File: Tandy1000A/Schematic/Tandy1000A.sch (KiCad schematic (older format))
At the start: 19 parts, among them J5 Floppy, U12 74LS138, U17 8259A, U25 VC2587/8079011 Custom, U26 74LS244, U28 8088, U31 74LS04, U41 74LS244, U51 BIOS ROM, U58 7417, U9 TACO111/3A-2125-BB/8079012 Cu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

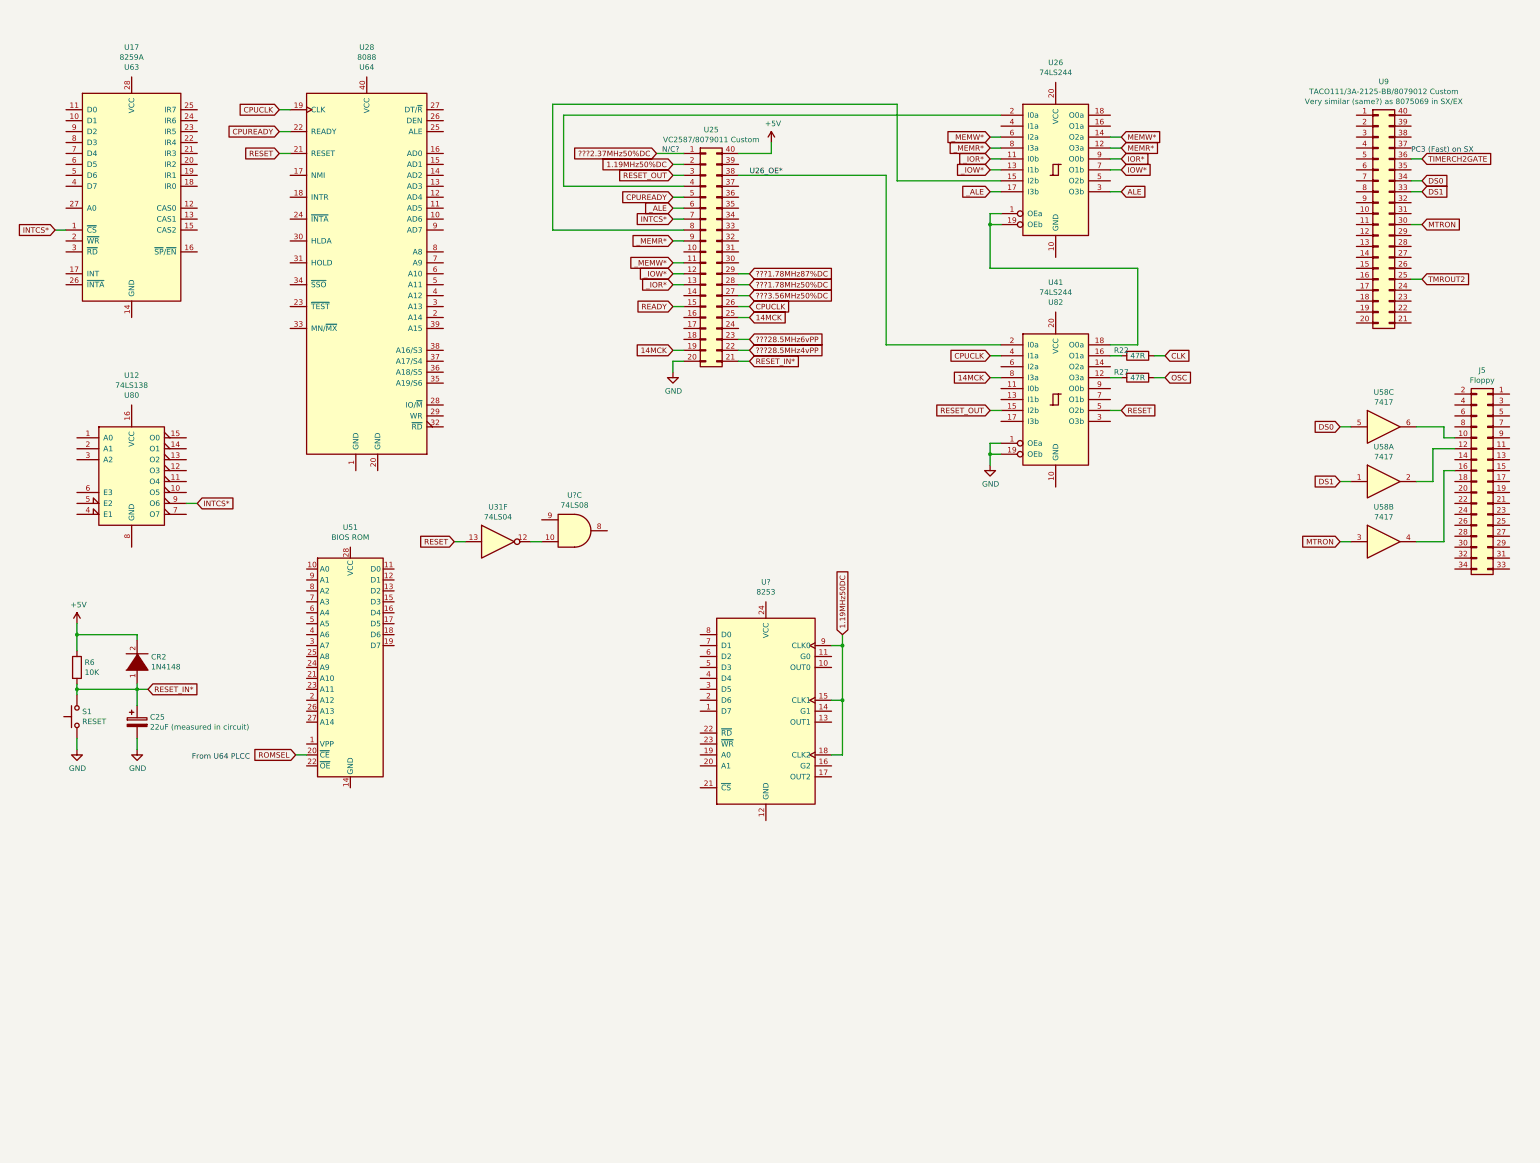
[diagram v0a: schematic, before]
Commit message: Readme and schematic updates.
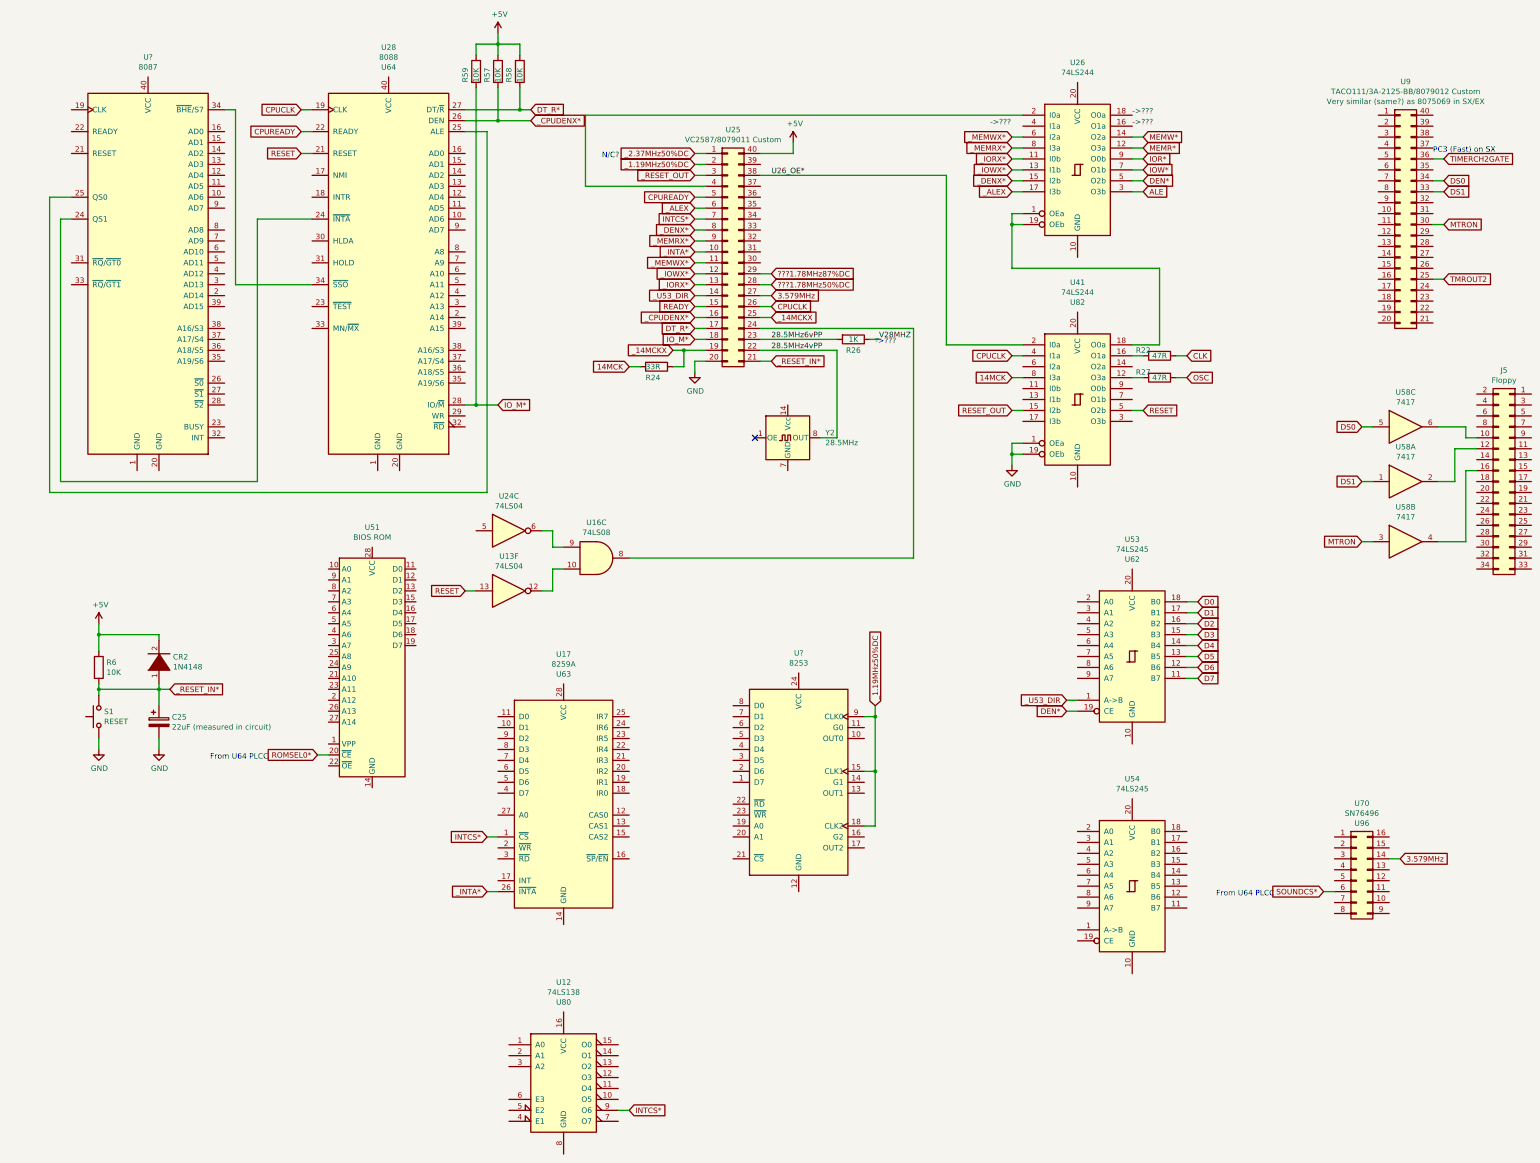
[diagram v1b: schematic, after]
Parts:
- added R24: 33R, symbol Device:R
- added R26: 1K, symbol Device:R
- added R57, R58, R59: 10K, symbol Device:R
- added U24: 74LS04, symbol 74xx:74LS04
- added U53, U54: 74LS245, symbol 74xx:74LS245
- added U70: SN76496, symbol Connector_Generic:Conn_02x08_Counter_Clockwise
- added U?: 8087, Package_DIP:DIP-40_W15.24mm, symbol MCU_Intel:8087
- added Y2: 28.5MHz, Oscillator:Oscillator_SeikoEpson_SG-8002DB, symbol Oscillator:SG-51
- gave numbers to parts that had none: 1
- renumbered U31 to U13
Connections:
- net 1.19MHz50DC is gone; now on net _1.19MHz50%DC: U?.15 (CLK1), U?.18 (CLK2), U?.9 (CLK0)
- net +5V: now also R57.1, R58.1, R59.1
- net 14MCK: now also R24.2; no longer U25.19 (Pin_19), U25.25 (Pin_25)
- net RESET_OUT: no longer U25.3 (Pin_3)
- net at U28.24 (~INTA~): now also U?.24 (QS1)
- net at U28.25 (ALE): now also U?.25 (QS0)
- net _CPUDENX*: now reaches U28.26 (DEN)
- net _CPUDENX*: now also U25.16 (Pin_16), R57.2
- net DT_R*: now reaches U28.27 (DT/~R~)
- net DT_R*: now also U25.17 (Pin_17), R58.2
- net IO_M*: now reaches U28.28 (IO/~M~)
- net IO_M*: now also U25.18 (Pin_18), R59.2
- net at U28.34 (~SSO~): now also U?.34 (~BHE~/S7)
- net at U16.8: now also U25.24 (Pin_24)
- net at U16.9: now also U24.6
- net _INTA*: now reaches U25.10 (Pin_10)
- net _INTA*: now also U17.26 (~INTA~)
- net _U53_DIR: now reaches U25.14 (Pin_14)
- net _U53_DIR: now also U53.1 (A->B)
- net _DENX*: now reaches U25.8 (Pin_8), U26.15 (I2b)
- net DEN*: now reaches U26.5 (O2b)
- net DEN*: now also U53.19 (CE)
- net 1.19MHz50%DC renamed _1.19MHz50%DC
- net ???2.37MHz50%DC renamed _2.37MHz50%DC
- net ???28.5MHz4vPP renamed 28.5MHz4vPP
- net 28.5MHz4vPP: now also Y2.8 (OUT)
- net ???28.5MHz6vPP renamed 28.5MHz6vPP
- net 28.5MHz6vPP: now also R26.2
- net ???3.56MHz50%DC renamed 3.579MHz
- net 3.579MHz: now also U70.14 (Pin_14)
- net RESET_IN* renamed _RESET_IN*
- net ROMSEL renamed ROMSEL0*
- net _ALE renamed _ALEX
- net _IOR* renamed _IORX*
- net _IOW* renamed _IOWX*
- net _MEMR* renamed _MEMRX*
- net _MEMW* renamed _MEMWX*
- new net D0: U53.18 (B0)
- new net D1: U53.17 (B1)
- new net D2: U53.16 (B2)
- new net D3: U53.15 (B3)
- new net D4: U53.14 (B4)
- new net D5: U53.13 (B5)
- new net D6: U53.12 (B6)
- new net D7: U53.11 (B7)
- new net SOUNDCS*: U70.6 (Pin_6)
- new net _14MCKX: R24.1, U25.19 (Pin_19), U25.25 (Pin_25)
- new net _RESET_OUT: U25.3 (Pin_3)
- new net _V28MHZ: R26.1
- no-connect marks 0 -> 1
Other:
- note added: "->???"
- moved on the sheet: C25, CR2, J5, R22, R27, R6, S1, U12, U13F, U16C, U17, U25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
